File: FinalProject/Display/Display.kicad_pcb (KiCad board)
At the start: 2 copper layers, 114.6 x 61.5 mm, 7 parts, among them J1 Conn_01x02_Pin, J5 Battery, M1 Stepper_Motor_bipolar

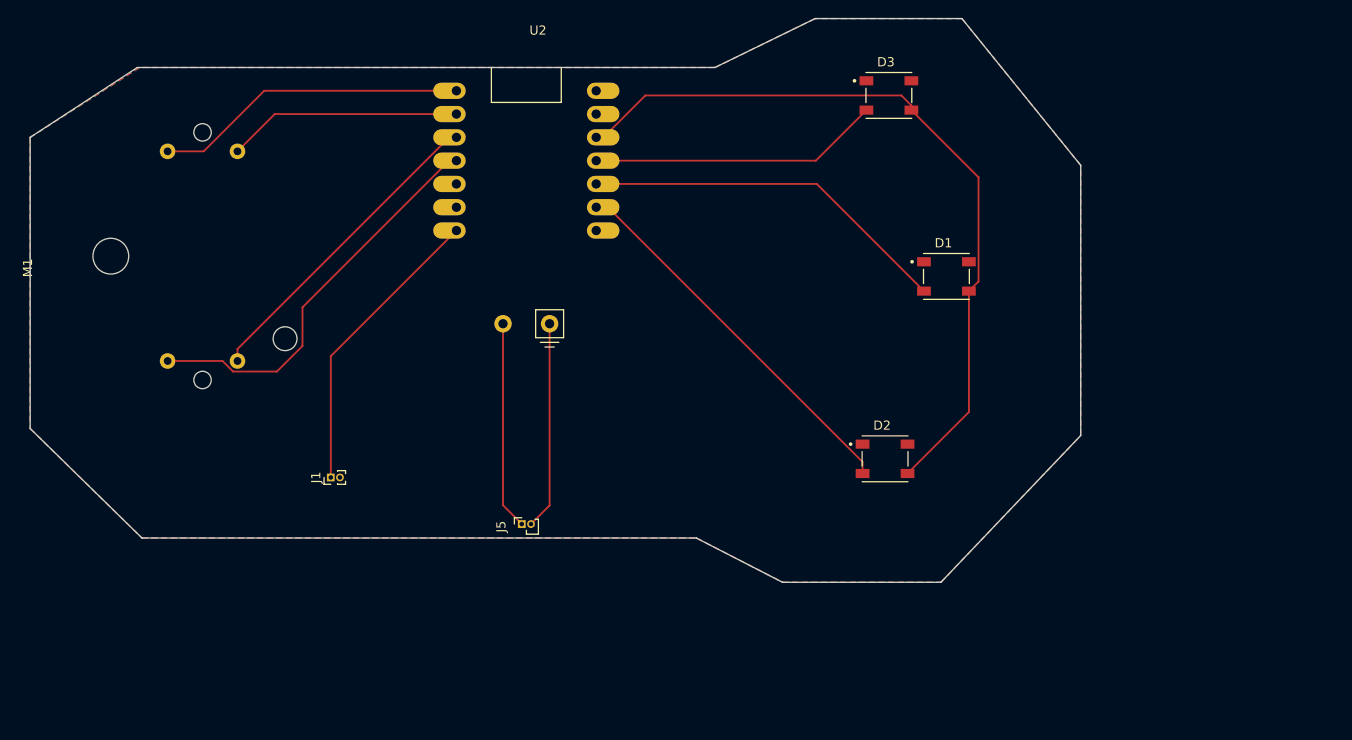
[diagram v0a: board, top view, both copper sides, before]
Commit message: Add pdf
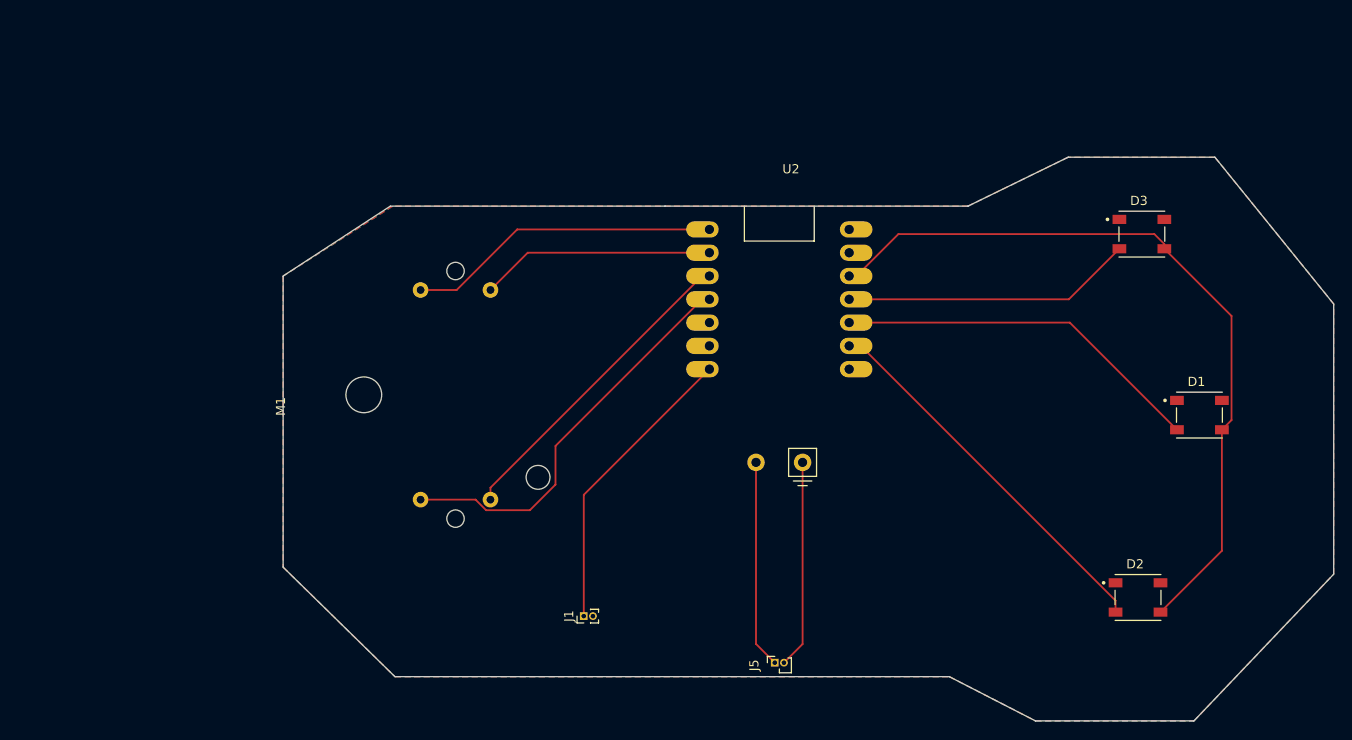
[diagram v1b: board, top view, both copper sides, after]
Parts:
- moved D1 31.5 mm to (196.8, 97.8)
- moved M1 31.5 mm to (125.9, 93.1)
- moved U2 31.5 mm to (151.0, 85.2)
- moved D2 31.5 mm to (190.1, 117.7)
- moved D3 31.5 mm to (190.6, 78.1)
- moved J1 31.5 mm to (129.7, 119.8)
- moved J5 31.5 mm to (150.5, 124.8)
